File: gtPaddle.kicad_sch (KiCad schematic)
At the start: 24 parts, among them IC1 74157N, IC2 74157N, Q14 2N3904, Q9 2N3904, U1 ADC0804LCN

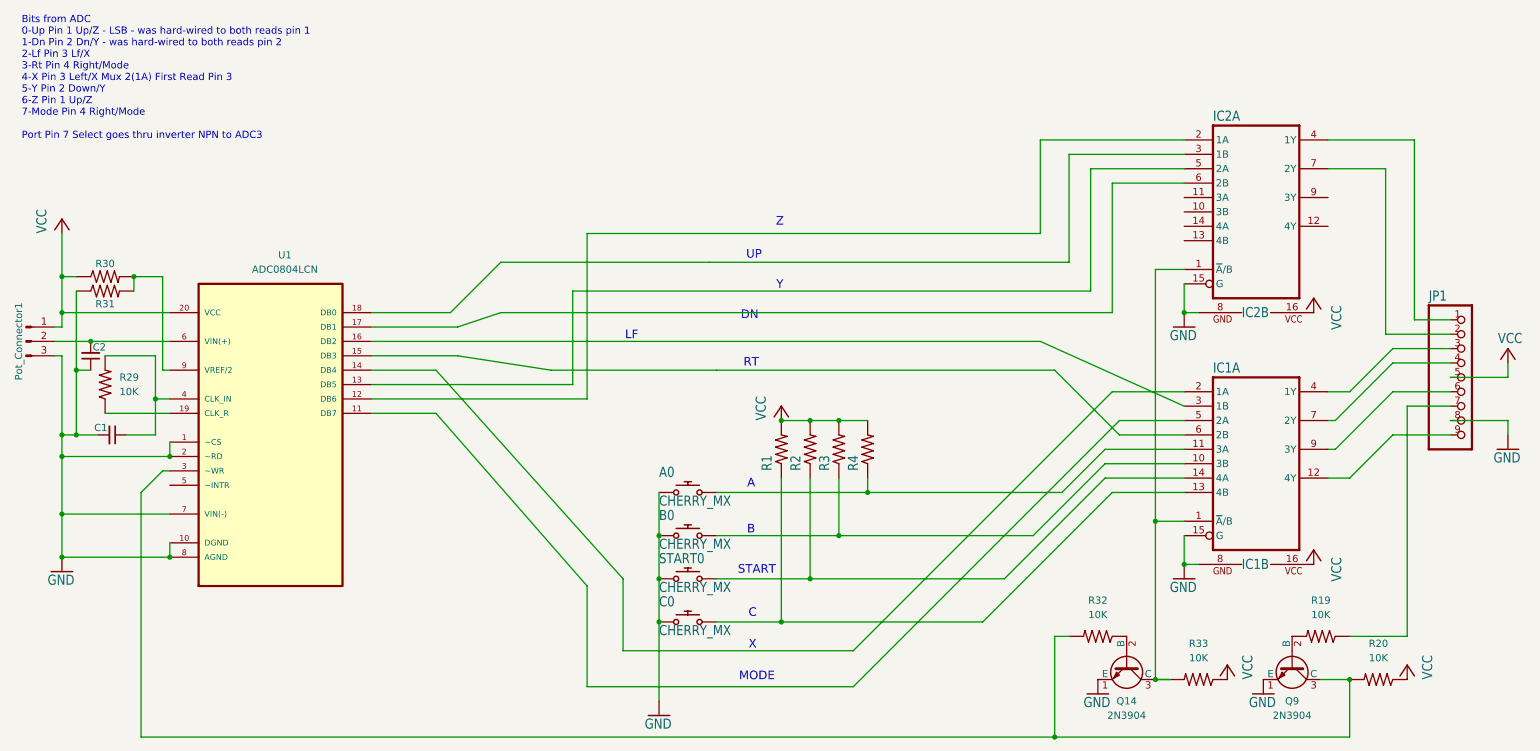
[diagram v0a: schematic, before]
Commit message: more simplified
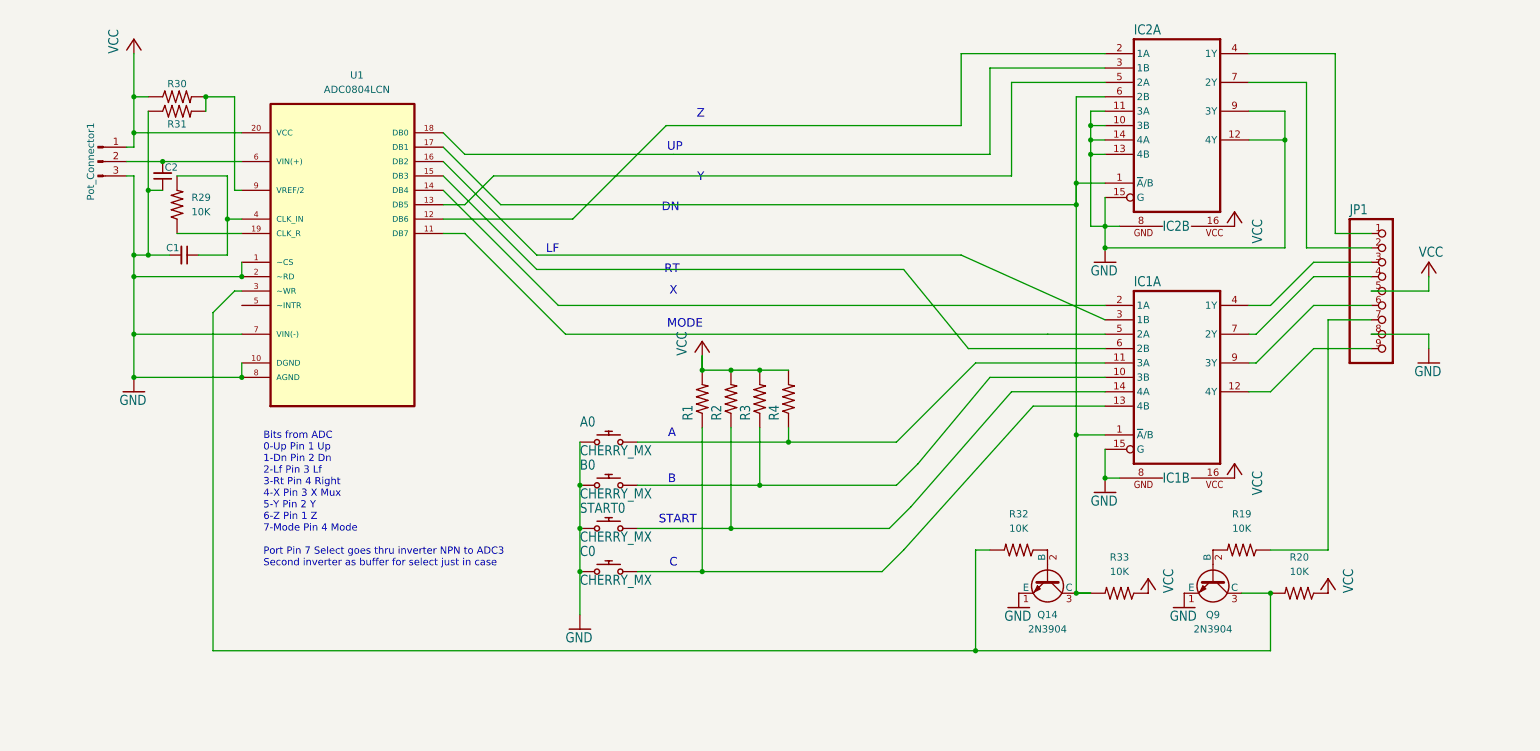
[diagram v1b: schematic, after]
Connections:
- net GND: now also IC2.10 (3B), IC2.11 (3A), IC2.12 (4Y), IC2.13 (4B), IC2.14 (4A), IC2.9 (3Y)
- net at IC1.1 (~{A}/B), IC2.1 (~{A}/B), Q14.3 (C)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: now also IC2.6 (2B), U1.17 (DB1)
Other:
- note added: "Bits from ADC 0-Up Pin 1 Up 1-Dn Pin 2 Dn 2-Lf Pin 3 Lf 3-Rt Pin 4 Right 4-X Pin 3 X Mux 5-Y Pin 2 Y 6-Z Pin 1 Z 7-Mode Pin 4 Mode Port Pin 7 Select goes thru inverter NPN to ADC3 Second inverter as buffer for select just in case"
- note removed: "Bits from ADC 0-Up Pin 1 Up/Z - LSB - was hard-wired to both reads pin 1 1-Dn Pin 2 Dn/Y - was hard-wired to both reads pin 2 2-Lf Pin 3 Lf/X 3-Rt Pin 4 Right/Mode 4-X Pin 3 Left/X Mux 2(1A) First Read Pin 3 5-Y Pin 2 Down/Y 6-Z Pin 1 Up/Z 7-Mode Pin 4 Right/Mode Port Pin 7 Select goes thru inverter NPN to ADC3"
- moved on the sheet: A0, B0, C0, C1, C2, IC1A, IC1B, IC2A, IC2B, JP1, Pot_Connector1, Q14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

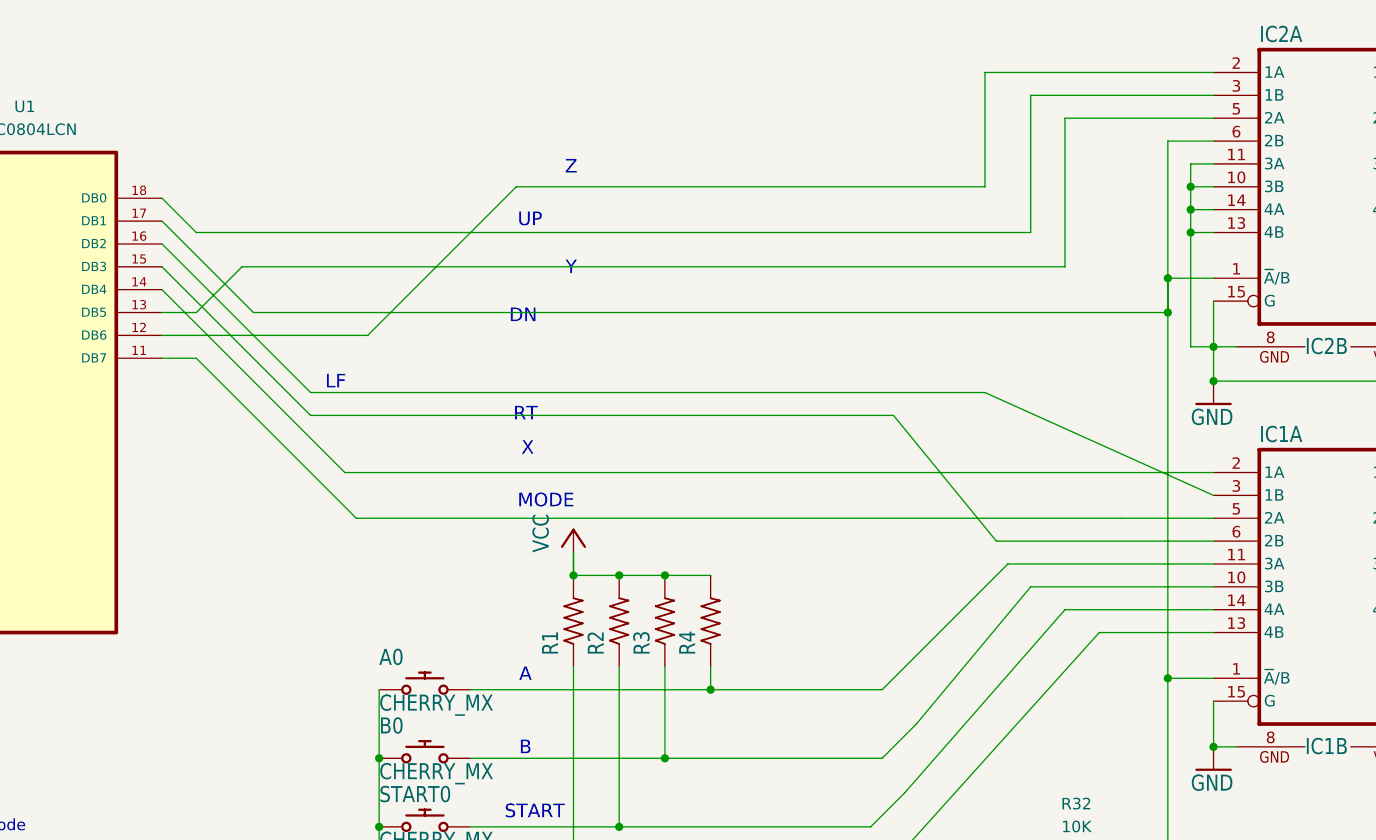
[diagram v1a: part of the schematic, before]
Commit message: some wire cleanup
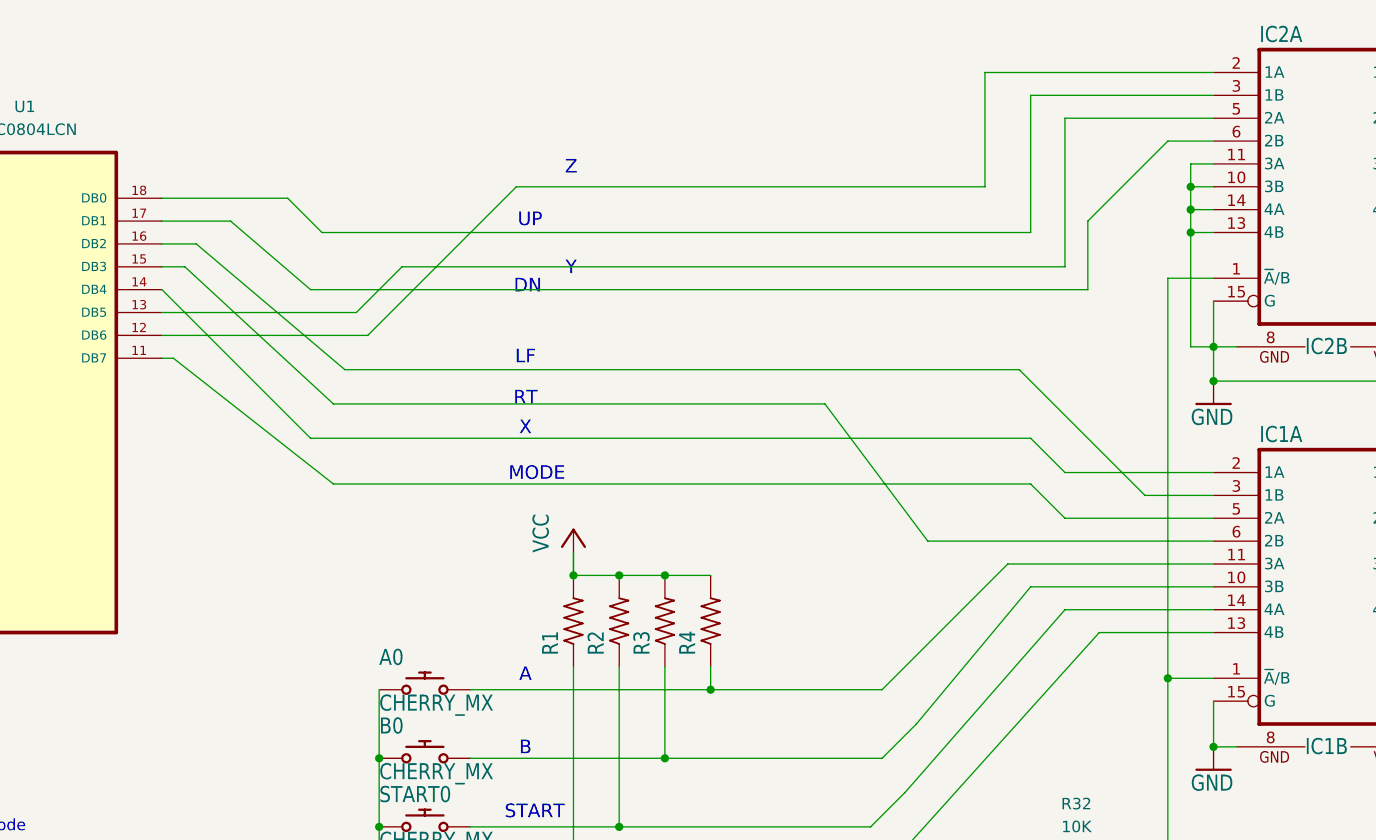
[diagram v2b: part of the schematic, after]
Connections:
- net at IC1.1 (~{A}/B), IC2.1 (~{A}/B), Q14.3 (C)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: no longer IC2.6 (2B), U1.17 (DB1)
- new net: IC2.6 (2B), U1.17 (DB1)
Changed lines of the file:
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@@
 	(text "MODE"
 		(exclude_from_sim no)
-		(at 136.652 88.392 0)
+		(at 135.636 85.344 0)
 		(effects
 			(font
@@
 	(text "RT"
 		(exclude_from_sim no)
-		(at 134.366 78.74 0)
+		(at 134.366 76.962 0)
 		(effects
 			(font
@@
 	(text "X"
 		(exclude_from_sim no)
-		(at 134.62 82.55 0)
+		(at 134.366 80.264 0)
 		(effects
 			(font
@@
 	(text "DN"
 		(exclude_from_sim no)
-		(at 134.112 67.818 0)
+		(at 134.62 64.516 0)
 		(effects
 			(font
@@
 	(text "LF"
 		(exclude_from_sim no)
-		(at 113.284 75.184 0)
+		(at 134.366 72.39 0)
 		(effects
 			(font
@@
 	)
 	(junction
-		(at 205.74 67.31)
-		(diameter 0)
-		(color 0 0 0 0)
-	)
-	(junction
 		(at 187.96 146.05)
 		(diameter 0)
@@
 	)
 	(junction
-		(at 205.74 63.5)
-		(diameter 0)
-		(color 0 0 0 0)
-	)
-	(junction
 		(at 118.11 124.46)
 		(diameter 0)
@@
 	(wire
 		(pts
+			(xy 196.85 64.77) (xy 196.85 57.15)
+		)
+		(stroke
+			(width 0)
+			(type default)
+		)
+	)
+	(wire
+		(pts
 			(xy 39.37 54.61) (xy 58.42 54.61)
 		)
@@
 	(wire
 		(pts
-			(xy 102.87 62.23) (xy 194.31 62.23)
+			(xy 120.65 62.23) (xy 194.31 62.23)
 		)
 		(stroke
@@
 	(wire
 		(pts
-			(xy 205.74 67.31) (xy 205.74 63.5)
+			(xy 190.5 86.36) (xy 194.31 90.17)
 		)
 		(stroke
@@
 	(wire
 		(pts
+			(xy 194.31 85.09) (xy 210.82 85.09)
+		)
+		(stroke
+			(width 0)
+			(type default)
+		)
+	)
+	(wire
+		(pts
 			(xy 240.03 100.33) (xy 247.65 92.71)
 		)
@@
 	(wire
 		(pts
-			(xy 114.3 85.09) (xy 93.98 64.77)
+			(xy 110.49 81.28) (xy 93.98 64.77)
 		)
 		(stroke
@@
 	(wire
 		(pts
+			(xy 196.85 57.15) (xy 205.74 48.26)
+		)
+		(stroke
+			(width 0)
+			(type default)
+		)
+	)
+	(wire
+		(pts
 			(xy 57.15 64.77) (xy 58.42 64.77)
 		)
@@
 	(wire
 		(pts
-			(xy 93.98 72.39) (xy 97.79 72.39)
+			(xy 93.98 72.39) (xy 95.25 72.39)
 		)
 		(stroke
@@
 	(wire
 		(pts
-			(xy 97.79 58.42) (xy 134.62 58.42)
+			(xy 111.76 58.42) (xy 134.62 58.42)
 		)
 		(stroke
@@
 	(wire
 		(pts
-			(xy 205.74 63.5) (xy 205.74 48.26)
-		)
-		(stroke
-			(width 0)
-			(type default)
-		)
-	)
-	(wire
-		(pts
 			(xy 194.31 62.23) (xy 194.31 45.72)
 		)
@@
 	(wire
 		(pts
-			(xy 110.49 78.74) (xy 93.98 62.23)
+			(xy 113.03 77.47) (xy 96.52 62.23)
 		)
 		(stroke
@@
 	(wire
 		(pts
-			(xy 97.79 58.42) (xy 93.98 54.61)
-		)
-		(stroke
-			(width 0)
-			(type default)
-		)
-	)
-	(wire
-		(pts
-			(xy 110.49 78.74) (xy 175.26 78.74)
+			(xy 111.76 58.42) (xy 107.95 54.61)
+		)
+		(stroke
+			(width 0)
+			(type default)
+		)
+	)
+	(wire
+		(pts
+			(xy 113.03 77.47) (xy 167.64 77.47)
 		)
 		(stroke
@@
 	(wire
 		(pts
-			(xy 205.74 67.31) (xy 205.74 107.95)
-		)
-		(stroke
-			(width 0.1524)
-			(type solid)
-		)
-	)
-	(wire
-		(pts
 			(xy 190.5 43.18) (xy 210.82 43.18)
 		)
@@
 	(wire
 		(pts
-			(xy 205.74 63.5) (xy 205.74 67.31)
+			(xy 205.74 63.5) (xy 205.74 107.95)
 		)
 		(stroke
@@
 	(wire
 		(pts
+			(xy 101.6 57.15) (xy 93.98 57.15)
+		)
+		(stroke
+			(width 0)
+			(type default)
+		)
+	)
+	(wire
+		(pts
+			(xy 194.31 85.09) (xy 190.5 81.28)
+		)
+		(stroke
+			(width 0)
+			(type default)
+		)
+	)
+	(wire
+		(pts
 			(xy 210.82 115.57) (xy 213.36 115.57)
 		)
@@
 	(wire
 		(pts
-			(xy 175.26 78.74) (xy 186.69 92.71)
+			(xy 167.64 77.47) (xy 179.07 92.71)
 		)
 		(stroke
@@
 	(wire
 		(pts
-			(xy 97.79 72.39) (xy 115.57 90.17)
+			(xy 95.25 72.39) (xy 113.03 86.36)
 		)
 		(stroke
@@
 	(wire
 		(pts
-			(xy 93.98 67.31) (xy 97.79 67.31)
+			(xy 93.98 67.31) (xy 115.57 67.31)
 		)
 		(stroke
@@
 	(wire
 		(pts
-			(xy 104.14 67.31) (xy 205.74 67.31)
+			(xy 110.49 64.77) (xy 196.85 64.77)
 		)
 		(stroke
@@
 	(wire
 		(pts
-			(xy 114.3 85.09) (xy 210.82 85.09)
+			(xy 110.49 81.28) (xy 190.5 81.28)
 		)
 		(stroke
@@
 	(wire
 		(pts
+			(xy 107.95 54.61) (xy 93.98 54.61)
+		)
+		(stroke
+			(width 0)
+			(type default)
+		)
+	)
+	(wire
+		(pts
 			(xy 234.95 135.89) (xy 240.03 135.89)
 		)
@@
 	(wire
 		(pts
-			(xy 104.14 67.31) (xy 93.98 57.15)
+			(xy 203.2 87.63) (xy 189.23 73.66)
+		)
+		(stroke
+			(width 0.1524)
+			(type solid)
+		)
+	)
+	(wire
+		(pts
+			(xy 110.49 64.77) (xy 101.6 57.15)
 		)
 		(stroke
@@
 	(wire
 		(pts
-			(xy 110.49 76.2) (xy 93.98 59.69)
-		)
-		(stroke
-			(width 0.1524)
-			(type solid)
-		)
-	)
-	(wire
-		(pts
-			(xy 200.66 90.17) (xy 210.82 90.17)
+			(xy 97.79 59.69) (xy 93.98 59.69)
+		)
+		(stroke
+			(width 0.1524)
+			(type solid)
+		)
+	)
+	(wire
+		(pts
+			(xy 114.3 73.66) (xy 97.79 59.69)
 		)
 		(stroke
@@
 	(wire
 		(pts
-			(xy 186.69 92.71) (xy 210.82 92.71)
-		)
-		(stroke
-			(width 0.1524)
-			(type solid)
-		)
-	)
-	(wire
-		(pts
-			(xy 115.57 90.17) (xy 200.66 90.17)
+			(xy 179.07 92.71) (xy 210.82 92.71)
+		)
+		(stroke
+			(width 0.1524)
+			(type solid)
+		)
+	)
+	(wire
+		(pts
+			(xy 113.03 86.36) (xy 190.5 86.36)
 		)
 		(stroke
@@
 	(wire
 		(pts
-			(xy 210.82 87.63) (xy 185.42 76.2)
-		)
-		(stroke
-			(width 0.1524)
-			(type solid)
-		)
-	)
-	(wire
-		(pts
 			(xy 144.78 106.68) (xy 144.78 124.46)
 		)
@@
 	(wire
 		(pts
-			(xy 97.79 67.31) (xy 102.87 62.23)
+			(xy 115.57 67.31) (xy 120.65 62.23)
 		)
 		(stroke
@@
 	(wire
 		(pts
-			(xy 110.49 76.2) (xy 185.42 76.2)
+			(xy 114.3 73.66) (xy 189.23 73.66)
 		)
 		(stroke
@@
 	(wire
 		(pts
+			(xy 203.2 87.63) (xy 210.82 87.63)
+		)
+		(stroke
+			(width 0.1524)
+			(type solid)
+		)
+	)
+	(wire
+		(pts
 			(xy 257.81 82.55) (xy 267.97 82.55)
 		)
@@
 	(wire
 		(pts
+			(xy 194.31 90.17) (xy 210.82 90.17)
+		)
+		(stroke
+			(width 0.1524)
+			(type solid)
+		)
+	)
+	(wire
+		(pts
 			(xy 44.45 59.69) (xy 58.42 59.69)
 		)
@@
 		)
 	)
+	(wire
+		(pts
+			(xy 96.52 62.23) (xy 93.98 62.23)
+		)
+		(stroke
+			(width 0.1524)
+			(type solid)
+		)
+	)
